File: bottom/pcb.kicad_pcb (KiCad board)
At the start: 2 copper layers, 99.1 x 90.2 mm, 24 parts, among them J1 Conn_01x01, J2 Conn_01x01, J3 Conn_01x01

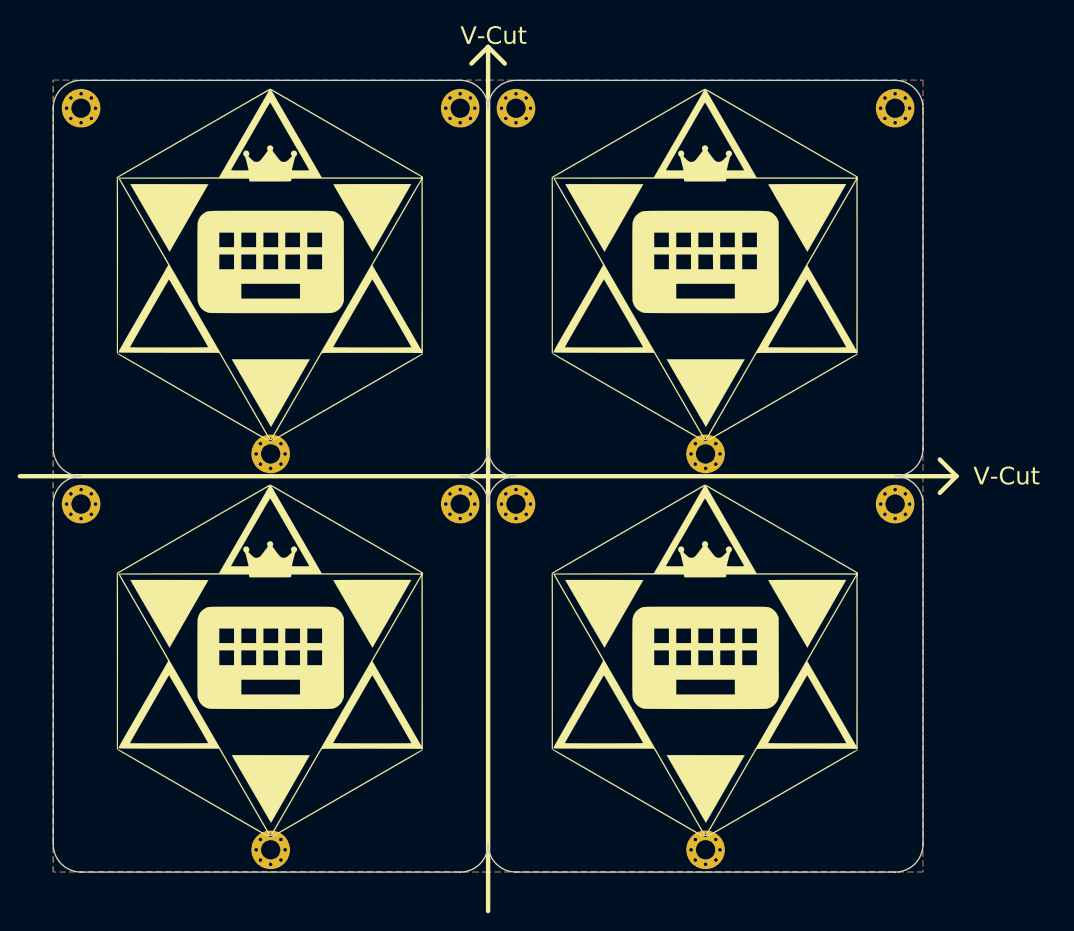
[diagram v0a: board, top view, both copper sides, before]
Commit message: create rubykaigi 2023
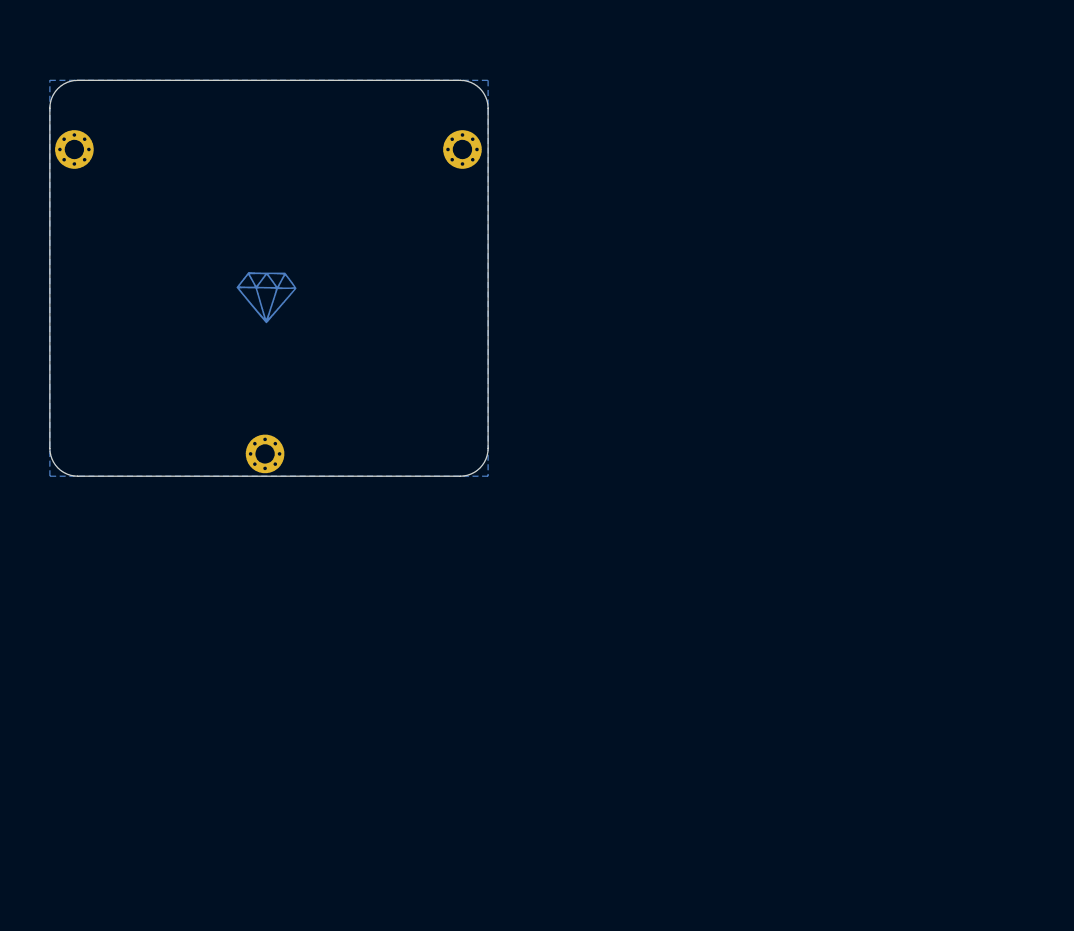
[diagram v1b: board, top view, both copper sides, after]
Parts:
- removed the G*** at (137.2, 116.2) (x2)
- removed the G*** at (137.2, 71.1) (x2)
- removed the G*** at (137.5, 70.8)
- removed the G*** at (137.5, 115.8)
- removed the G*** at (87.6, 116.2) (x2)
- removed the G*** at (87.9, 115.8)
- removed the G*** at (87.6, 71.1) (x2)
- removed the G*** at (87.9, 70.8)
- removed the J1 at (115.6, 98.4)
- removed the J1 at (66.0, 98.4)
- removed the J1 at (115.6, 53.3)
- removed the J2 at (137.2, 137.8)
- removed the J2 at (87.6, 137.8)
- removed the J2 at (137.2, 92.7)
- removed the J3 at (158.8, 53.3)
- removed the J3 at (158.8, 98.4)
- removed the J3 at (109.2, 98.4)
- added G***: LOGO, rubykaigi:logo_black, B.Cu at (87.0, 74.9)
- added G***: LOGO, rubykaigi:logo_ruby-mask, B.Cu at (87.0, 74.9)
- added G***: LOGO, rubykaigi:logo_ruby-cu, B.Cu at (87.0, 74.9)
- added G***: LOGO, rubykaigi:logo_silver, B.Cu at (87.0, 74.9)
- moved J1 4.76 mm to (65.3, 58.0)
- moved J3 4.71 mm to (109.5, 58.0)
- moved J2 0.63 mm to (87.0, 92.7)
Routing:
- removed copper zone on F.Cu, net GND
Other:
- board size 99.1 x 90.2 mm -> 49.9 x 45.1 mm
- net class Default removed
- net class PWR removed
- board text removed: "V-Cut"
